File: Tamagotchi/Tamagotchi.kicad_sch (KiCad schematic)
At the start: 4 parts, among them J1 Conn_01x20, J2 Conn_01x20, J3 Conn_01x06, J4 Conn_01x07

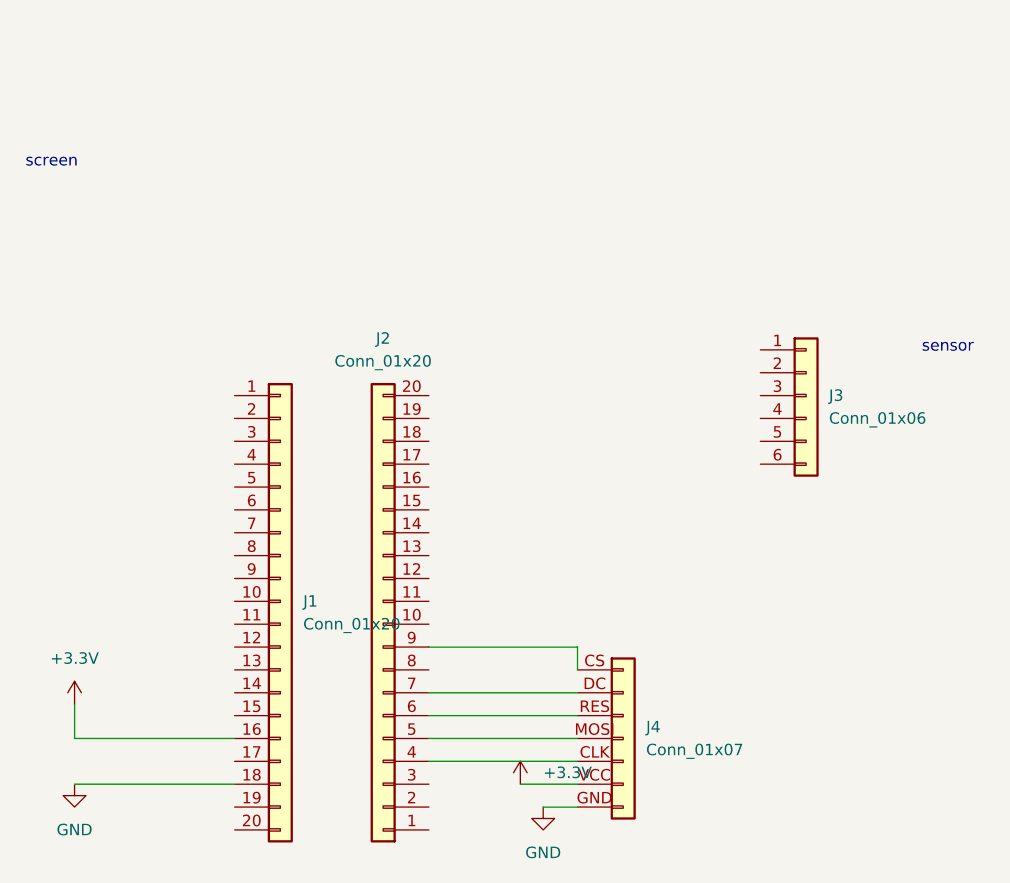
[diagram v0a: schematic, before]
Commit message: schematic updated
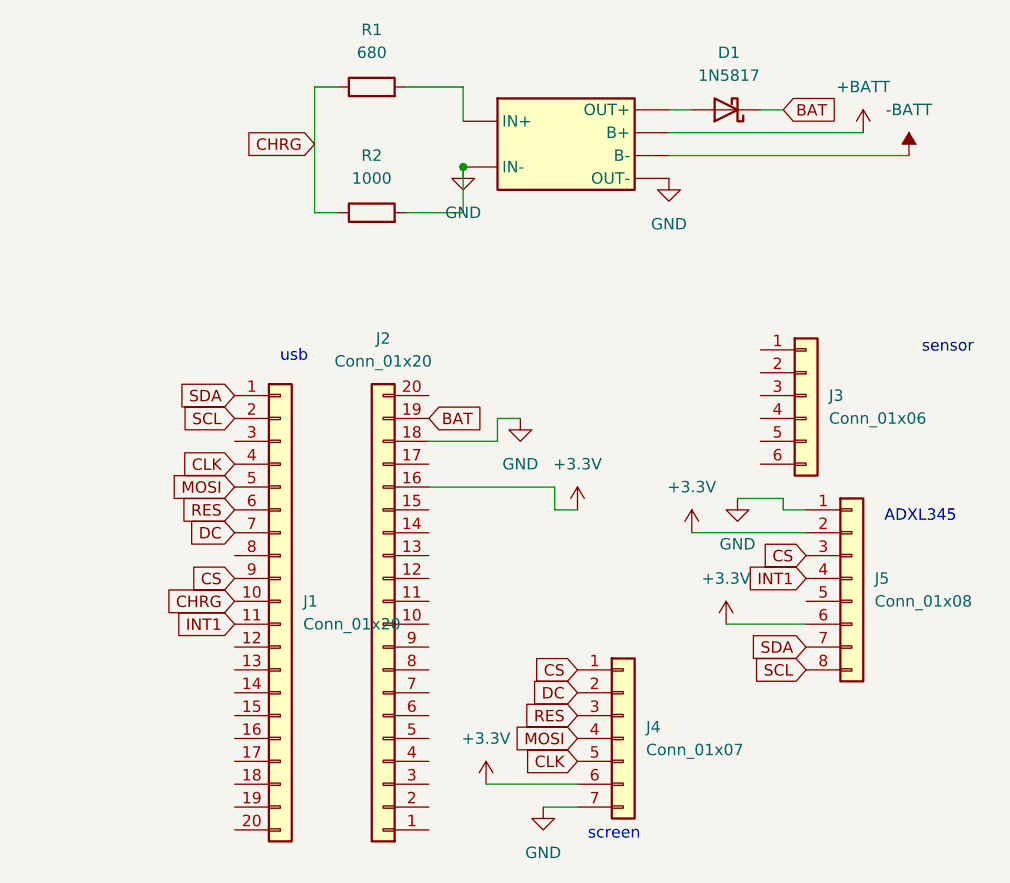
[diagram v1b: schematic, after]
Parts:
- added D1: 1N5817, Diode_THT:D_DO-41_SOD81_P10.16mm_Horizontal, symbol Diode:1N5817
- added J5: Conn_01x08, symbol Connector_Generic:Conn_01x08
- added R1: 680, symbol Device:R
- added R2: 1000, symbol Device:R
- added U1: TP4056-module, Package_SO:SOIC-8-1EP_3.9x4.9mm_P1.27mm_EP2.41x3.3mm_ThermalVias, symbol Tama_Symbols:TP4056-MODULE
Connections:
- net +3.3V: now also J2.16 (Pin_16), J4.6 (Pin_6), J5.2 (Pin_2), J5.6 (Pin_6); no longer J1.16 (Pin_16), J4.VCC (Pin_6)
- net GND: now also J2.18 (Pin_18), J4.7 (Pin_7), J5.1 (Pin_1), R2.2, U1. (OUT-); no longer J1.18 (Pin_18), J4.GND (Pin_7)
- net BAT: now reaches J2.19 (Pin_19)
- net BAT: now also D1.1 (K)
- net at J2.4 (Pin_4): no longer J4.CLK (Pin_5)
- net at J2.5 (Pin_5): no longer J4.MOSI (Pin_4)
- net at J2.6 (Pin_6): no longer J4.RES (Pin_3)
- net at J2.7 (Pin_7): no longer J4.DC (Pin_2)
- net at J2.9 (Pin_9): no longer J4.CS (Pin_1)
- net SDA: now reaches J1.1 (Pin_1)
- net SDA: now also J5.7 (Pin_7)
- net CHRG: now reaches J1.10 (Pin_10)
- net CHRG: now also R1.1, R2.1
- net INT1: now reaches J1.11 (Pin_11)
- net INT1: now also J5.4 (Pin_4)
- net SCL: now reaches J1.2 (Pin_2)
- net SCL: now also J5.8 (Pin_8)
- net CLK: now reaches J1.4 (Pin_4)
- net CLK: now also J4.5 (Pin_5)
- net MOSI: now reaches J1.5 (Pin_5)
- net MOSI: now also J4.4 (Pin_4)
- net RES: now reaches J1.6 (Pin_6)
- net RES: now also J4.3 (Pin_3)
- net DC: now reaches J1.7 (Pin_7)
- net DC: now also J4.2 (Pin_2)
- net CS: now reaches J1.9 (Pin_9)
- net CS: now also J4.1 (Pin_1), J5.3 (Pin_3)
- new net: D1.2 (A), U1. (OUT-)
- new net: R1.2, U1. (OUT-)
- new net +BATT: U1. (OUT-)
- new net -BATT: U1. (OUT-)
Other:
- note added: "ADXL345"
- note added: "usb"
- moved on the sheet: J4
